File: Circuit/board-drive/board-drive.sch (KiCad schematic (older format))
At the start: 29 parts, among them P1 XT30, P10 XT60, P2 XT30, P3 XT30, P4 XT30, P5 XT30, P6 XT30, P7 XT30, P8 XT30, P9 XT60, U1 Pololu_Maestro12, U10 PowerDist_WiretoBoard, U11 PowerDist_WiretoBoard, U12 Pololu_SimpleMotorController2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, U13 Pololu_SimpleMotorController2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, U14 Pololu_SimpleMotorController2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, U15 Pololu_SimpleMotorController2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, U16 PowerDist_WiretoBoard, U17 PowerDist_WiretoBoard, U18 PowerDist_WiretoBoard, U19 PowerDist_WiretoBoard, U2 Si8660BA-B-IS1, U3 Si8660BA-B-IS1, U4 Pololu_SimpleMotorController2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, U5 Pololu_SimpleMotorController2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, U6 Pololu_SimpleMotorController2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, U7 Pololu_SimpleMotorController2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, U8 PowerDist_WiretoBoard, U9 PowerDist_WiretoBoard

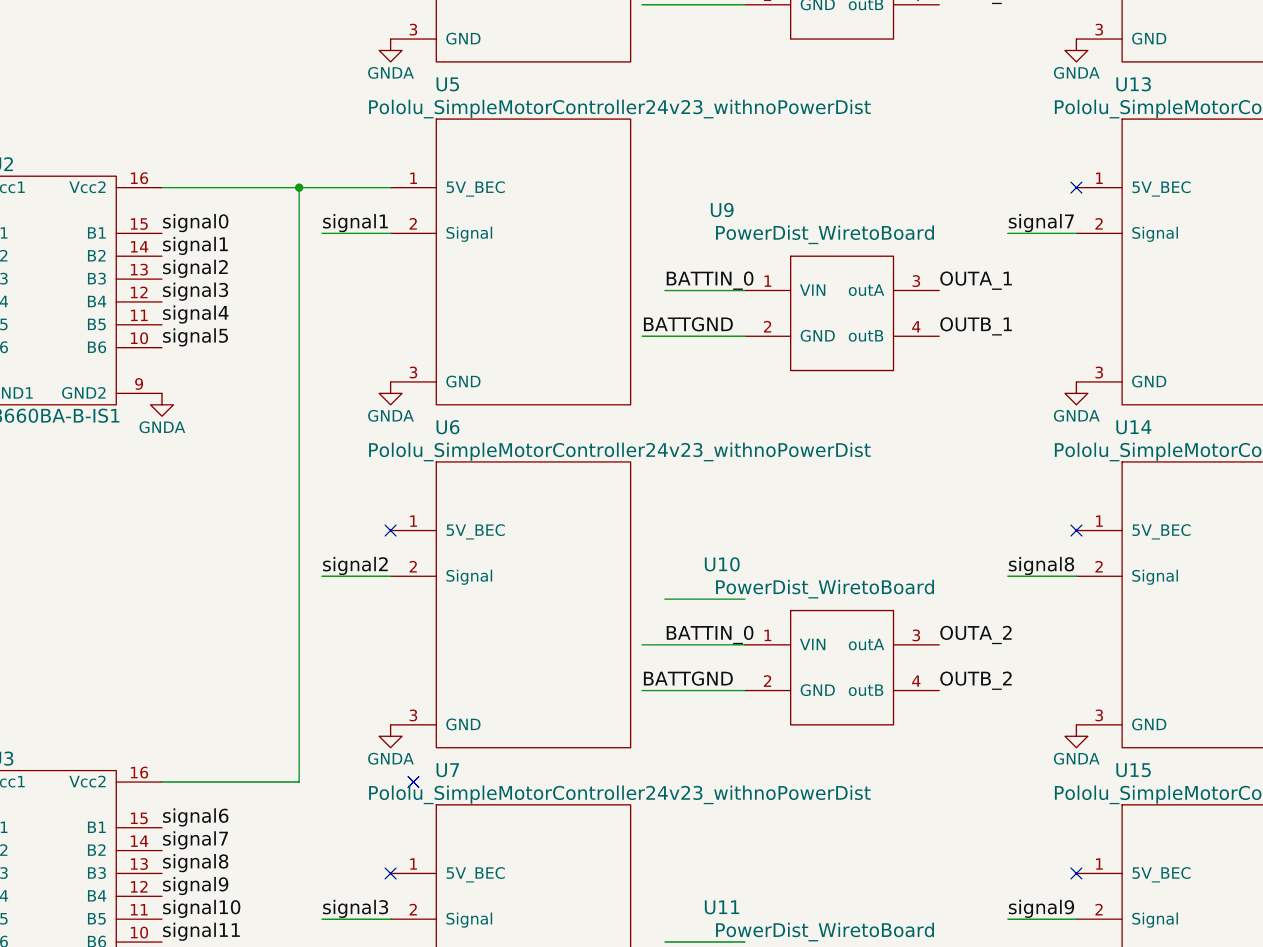
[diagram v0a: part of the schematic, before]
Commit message: edited sch and pcb
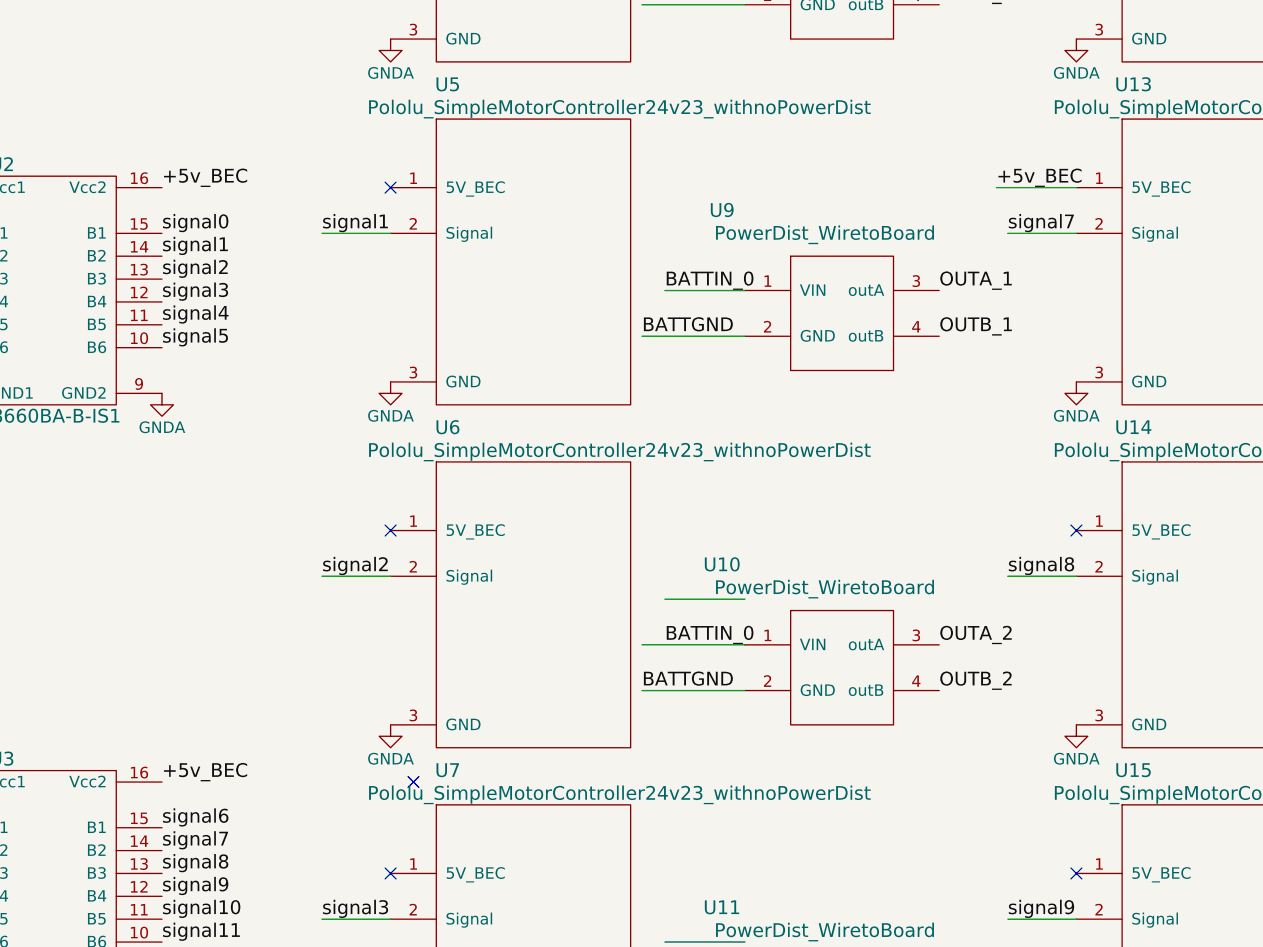
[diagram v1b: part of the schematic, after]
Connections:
- net labels added: +5v_BEC
- wire segments 89 -> 87
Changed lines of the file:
@@
 NoConn ~ 8250 5500
 NoConn ~ 8250 4000
-NoConn ~ 8250 2500
 NoConn ~ 8250 1000
 NoConn ~ 5350 5100
@@
 Wire Wire Line
 	6800 6200 6350 6200
-Wire Wire Line
-	4250 2500 5250 2500
-Wire Wire Line
-	4850 2500 4850 5100
-Wire Wire Line
-	4850 5100 4250 5100
-Connection ~ 4850 2500
+Text Label 4250 2500 0    60   ~ 0
++5v_BEC
+Text Label 4250 5100 0    60   ~ 0
++5v_BEC
+Text Label 7900 2500 0    60   ~ 0
++5v_BEC
+Wire Wire Line
+	7900 2500 8250 2500
+NoConn ~ 5250 2500
 $EndSCHEMATC
